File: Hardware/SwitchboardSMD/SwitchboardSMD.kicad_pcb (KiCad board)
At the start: 2 copper layers, 70 x 40 mm, 40 parts, among them J2 S88_In_Plug, J4 S88_Out_Plug, Q1 BC237, SW1 SW_Push, SW2 SW_Push, SW3 SW_Push, SW4 SW_Push, SW5 SW_Push, SW6 SW_Push, SW7 SW_Push, SW8 SW_Push, U1 4044, U2 4044, U3 4014

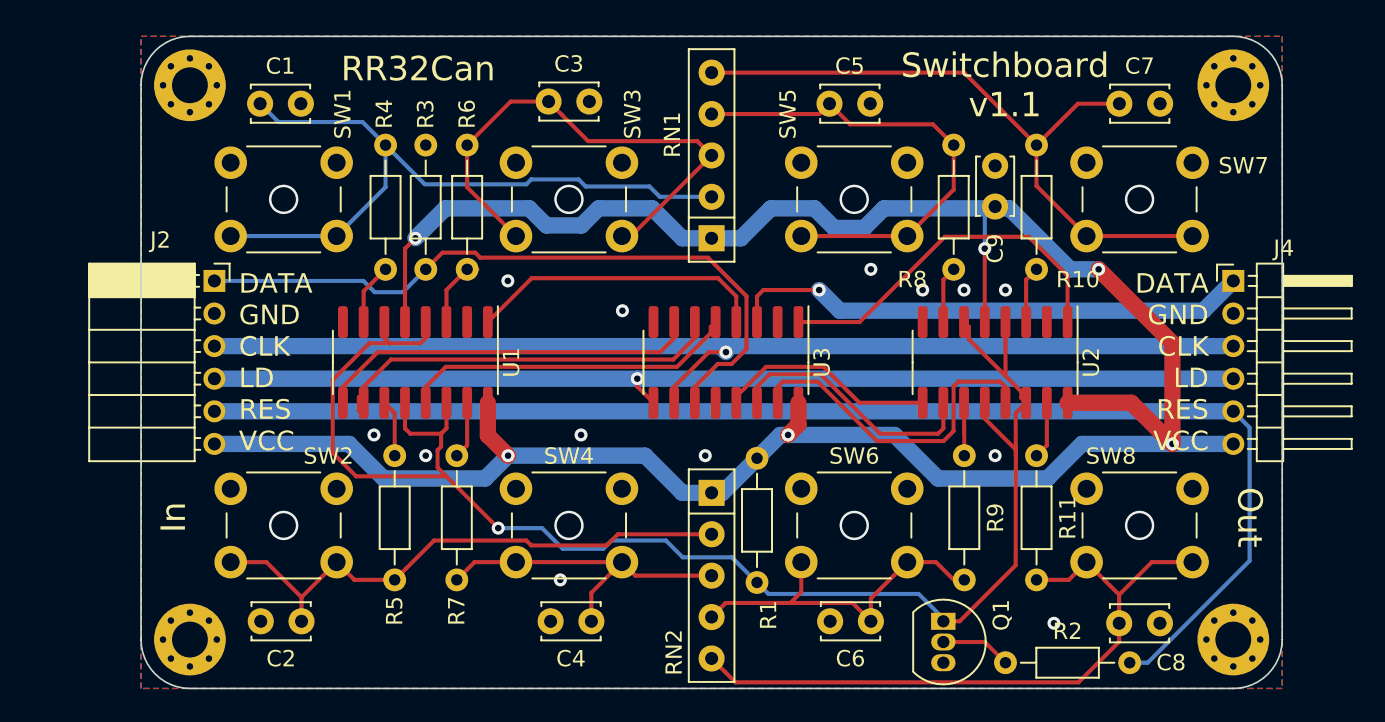
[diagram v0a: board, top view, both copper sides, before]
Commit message: Updated to v1.3 for manufacturing
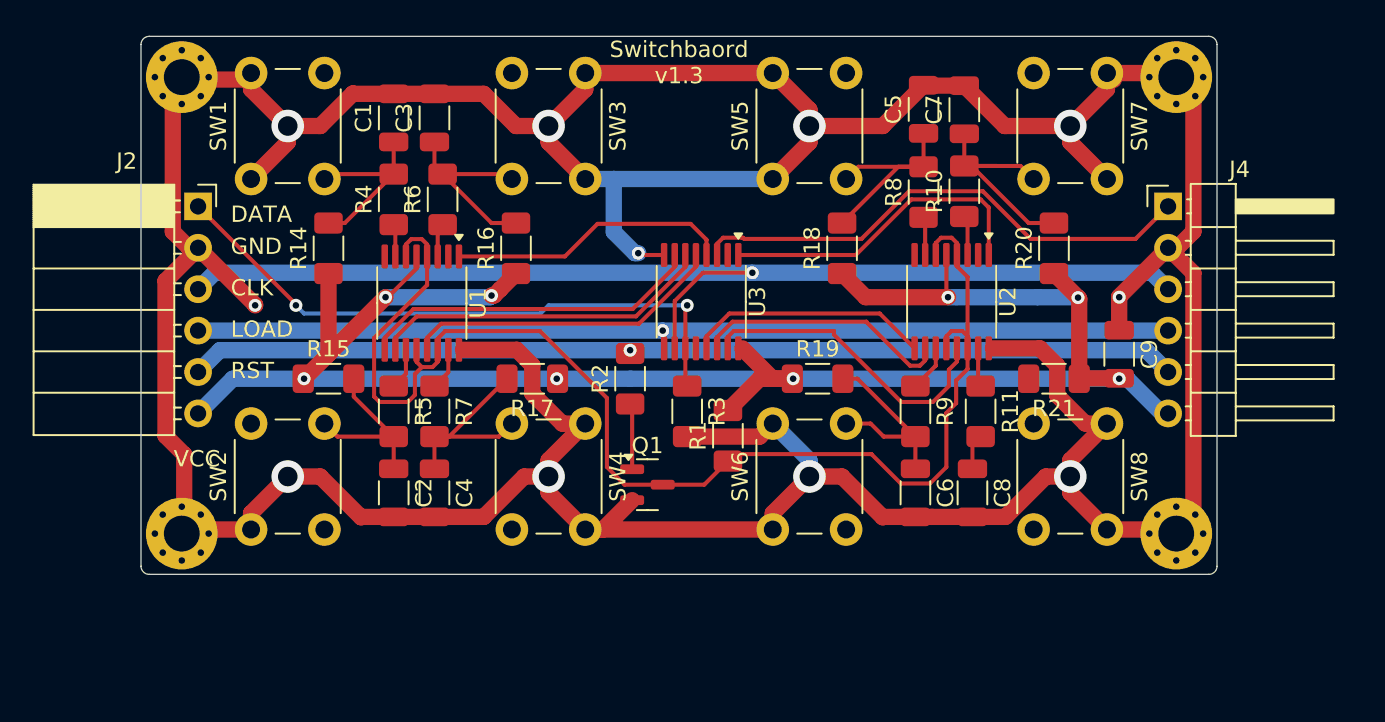
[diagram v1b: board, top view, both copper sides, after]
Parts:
- removed RN1, RN2: 100k, Resistor_THT:R_Array_SIP5
- added R14: 100k, Resistor_SMD:R_1206_3216Metric_Pad1.30x1.75mm_HandSolder, F.Cu at (31.5, 33.0)
- added R15: 100k, Resistor_SMD:R_1206_3216Metric_Pad1.30x1.75mm_HandSolder, F.Cu at (31.5, 41.0)
- added R16: 100k, Resistor_SMD:R_1206_3216Metric_Pad1.30x1.75mm_HandSolder, F.Cu at (43.0, 33.0)
- added R17: 100k, Resistor_SMD:R_1206_3216Metric_Pad1.30x1.75mm_HandSolder, F.Cu at (44.0, 41.0)
- added R18: 100k, Resistor_SMD:R_1206_3216Metric_Pad1.30x1.75mm_HandSolder, F.Cu at (63.0, 33.0)
- added R19: 100k, Resistor_SMD:R_1206_3216Metric_Pad1.30x1.75mm_HandSolder, F.Cu at (61.5, 41.0)
- added R20: 100k, Resistor_SMD:R_1206_3216Metric_Pad1.30x1.75mm_HandSolder, F.Cu at (76.0, 33.0)
- added R21: 100k, Resistor_SMD:R_1206_3216Metric_Pad1.30x1.75mm_HandSolder, F.Cu at (76.0, 41.0)
- C1, C2, C3, C4, C5, C6, C7, C8, C9: footprint Capacitor_THT:C_Disc_D3.4mm_W2.1mm_P2.50mm -> Capacitor_SMD:C_1206_3216Metric
- J2: footprint Connector_PinSocket_2.00mm:PinSocket_1x06_P2.00mm_Horizontal -> Connector_PinSocket_2.54mm:PinSocket_1x06_P2.54mm_Horizontal
- J4: footprint Connector_PinHeader_2.00mm:PinHeader_1x06_P2.00mm_Horizontal -> Connector_PinHeader_2.54mm:PinHeader_1x06_P2.54mm_Horizontal
- Q1: value BC237 -> MMBT5551L; footprint Package_TO_SOT_THT:TO-92_Inline -> Package_TO_SOT_SMD:SOT-23
- R1, R10, R11, R2, R3, R4, R5, R6, R7, R8, R9: footprint Resistor_THT:R_Axial_DIN0204_L3.6mm_D1.6mm_P7.62mm_Horizontal -> Resistor_SMD:R_1206_3216Metric_Pad1.30x1.75mm_HandSolder
- U1, U2, U3: footprint Package_SO:SOIC-16_3.9x9.9mm_P1.27mm -> Package_SO:TSSOP-16_4.4x5mm_P0.65mm
- moved H4 66.5 mm to (83.5, 50.5)
- moved H2 64.8 mm to (22.5, 50.5)
- moved H1 34.5 mm to (22.5, 22.5)
- moved R2 28.9 mm to (50.0, 41.0), turned to 90 degrees
- moved Q1 20.0 mm to (51.1, 47.5), turned to 0 degrees
- moved R3 18.2 mm to (53.5, 43.0), turned to -90 degrees
- moved C9 13.8 mm to (80.0, 39.5)
- moved C4 12.4 mm to (38.0, 48.0), turned to -90 degrees
- moved C8 12.0 mm to (71.0, 48.0), turned to -90 degrees
- moved C2 9.70 mm to (35.5, 48.0), turned to -90 degrees
- moved C7 9.52 mm to (70.5, 24.5), turned to 90 degrees
- moved R1 9.18 mm to (56.0, 44.5)
- moved C6 8.34 mm to (67.5, 48.0), turned to -90 degrees
- moved C1 8.24 mm to (35.5, 25.0), turned to 90 degrees
- moved C3 7.07 mm to (38.0, 25.0), turned to 90 degrees
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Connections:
- Q1 pad 1: /RESET_LOCAL -> Net-(Q1-C)
- Q1 pad 2: Net-(Q1-Pad2) -> GND
- Q1 pad 3: GND -> /RESET_LOCAL
- R2 pad 1: Net-(Q1-Pad2) -> Net-(Q1-C)
- U1 pad 16: VCC -> GND
- U1 pad 8: GND -> unconnected-(U1-Vss-Pad8)
- U2 pad 16: VCC -> GND
- U2 pad 8: GND -> unconnected-(U2-Vss-Pad8)
- U3 pad 12: (no net) -> unconnected-(U3-Q6-Pad12)
- U3 pad 2: (no net) -> unconnected-(U3-Q5-Pad2)
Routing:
- net GND: track 0.00 -> 298.6 mm, vias 21 -> 11
- net Net-(C8-Pad1): track 41.2 -> 1.98 mm
- net VCC: track 153.9 -> 121.2 mm, vias 6 -> 8
- net Net-(C1-Pad1): track 43.6 -> 11.6 mm
- net Net-(C7-Pad1): track 41.3 -> 15.5 mm
- net Net-(C2-Pad1): track 34.6 -> 11.1 mm
- net /RESET: track 82.0 -> 60.6 mm, vias 0 -> 1
- net Net-(C3-Pad1): track 31.8 -> 12.3 mm
- net Net-(C5-Pad1): track 29.4 -> 13.5 mm
- net /RESET_LOCAL: track 94.9 -> 81.0 mm, vias 1 -> 0
- net Net-(C6-Pad1): track 21.2 -> 12.5 mm
- net Net-(C4-Pad1): track 21.6 -> 13.0 mm
- net /DATA_IN: track 43.4 -> 38.0 mm, vias 0 -> 2
- net /LOAD: track 65.6 -> 60.6 mm
- net Net-(U3-P1): track 25.6 -> 21.1 mm
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- removed copper zone on B.Cu, net GND
- removed copper zone on F.Cu, net GND
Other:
- board size 70 x 40 mm -> 66 x 33 mm
- net class Default removed
- net class Power removed
- board text added: "CLK"
- board text added: "DATA"
- board text added: "GND"
- board text added: "LOAD"
- board text added: "RST"
- board text added: "Switchbaord v1.3"
- board text added: "VCC"
- board text removed: "DATA GND CLK LD RES VCC"
- board text removed: "In"
- board text removed: "Out"
- board text removed: "RR32Can"
- board text removed: "Switchboard v1.1"
